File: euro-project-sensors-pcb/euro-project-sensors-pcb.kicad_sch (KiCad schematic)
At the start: 25 parts, among them J1 CH0, J2 CH0, J3 CH0, J4 CH0

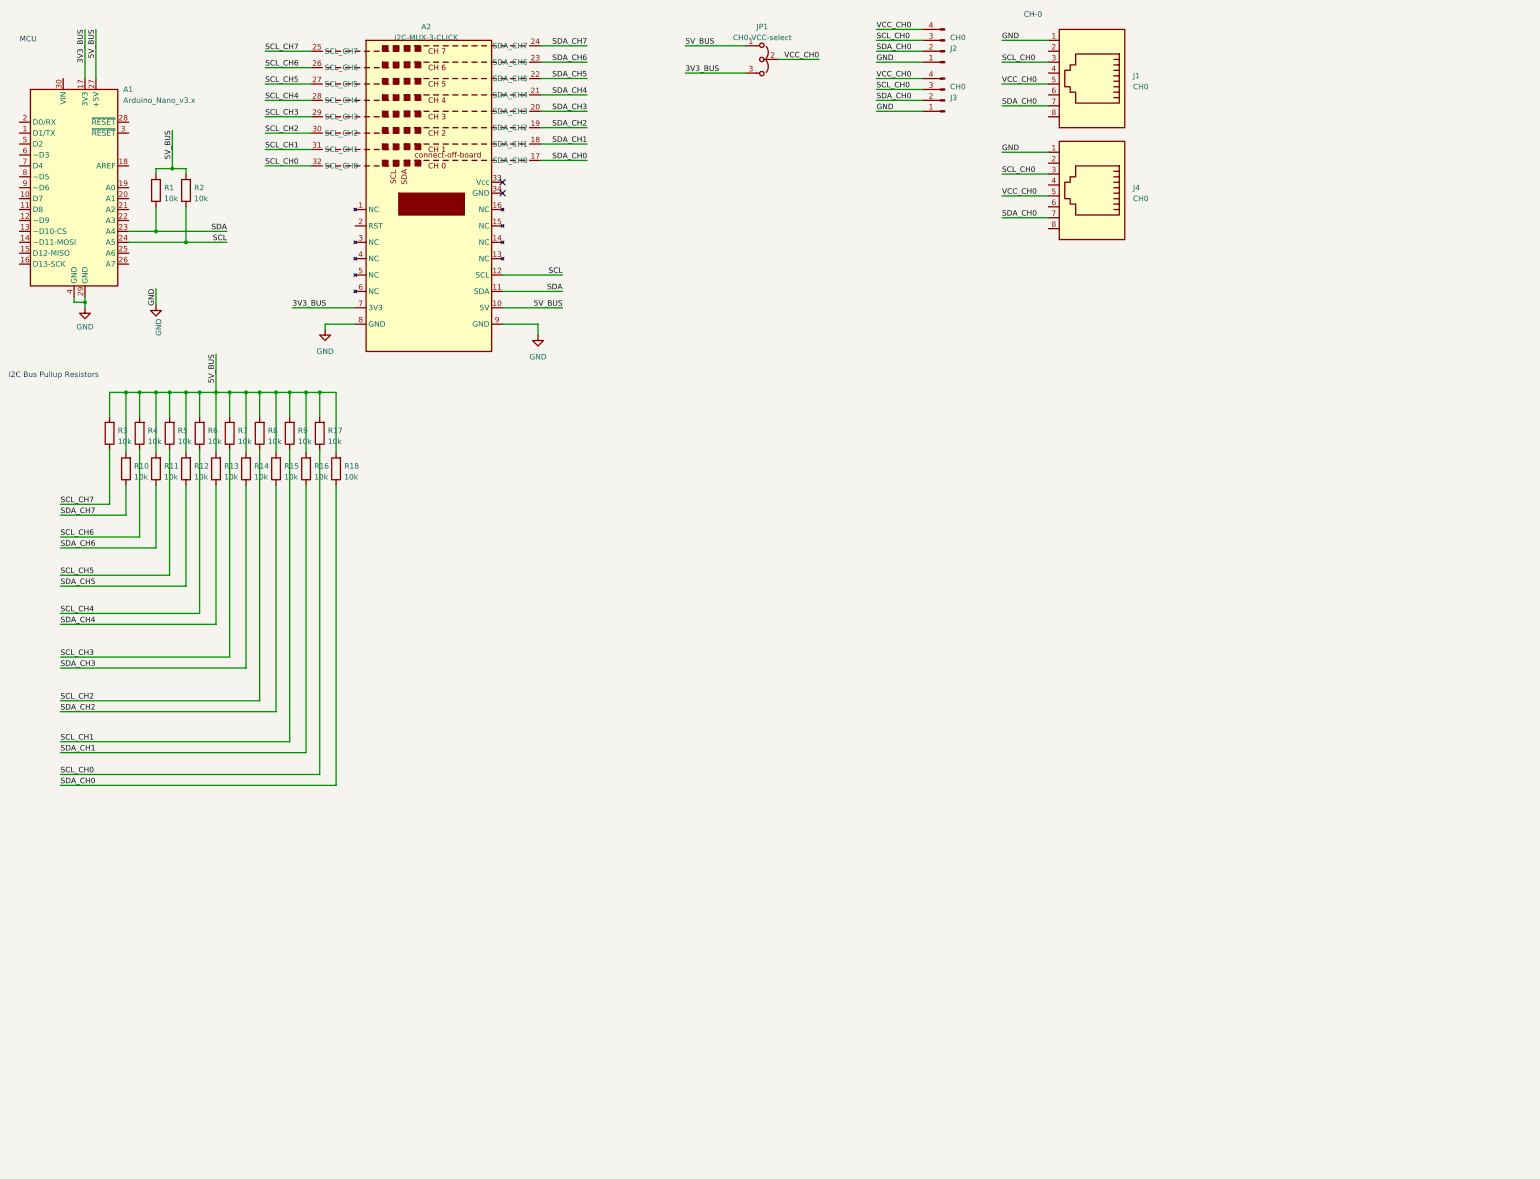
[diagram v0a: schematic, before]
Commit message: dfgbdfbdb
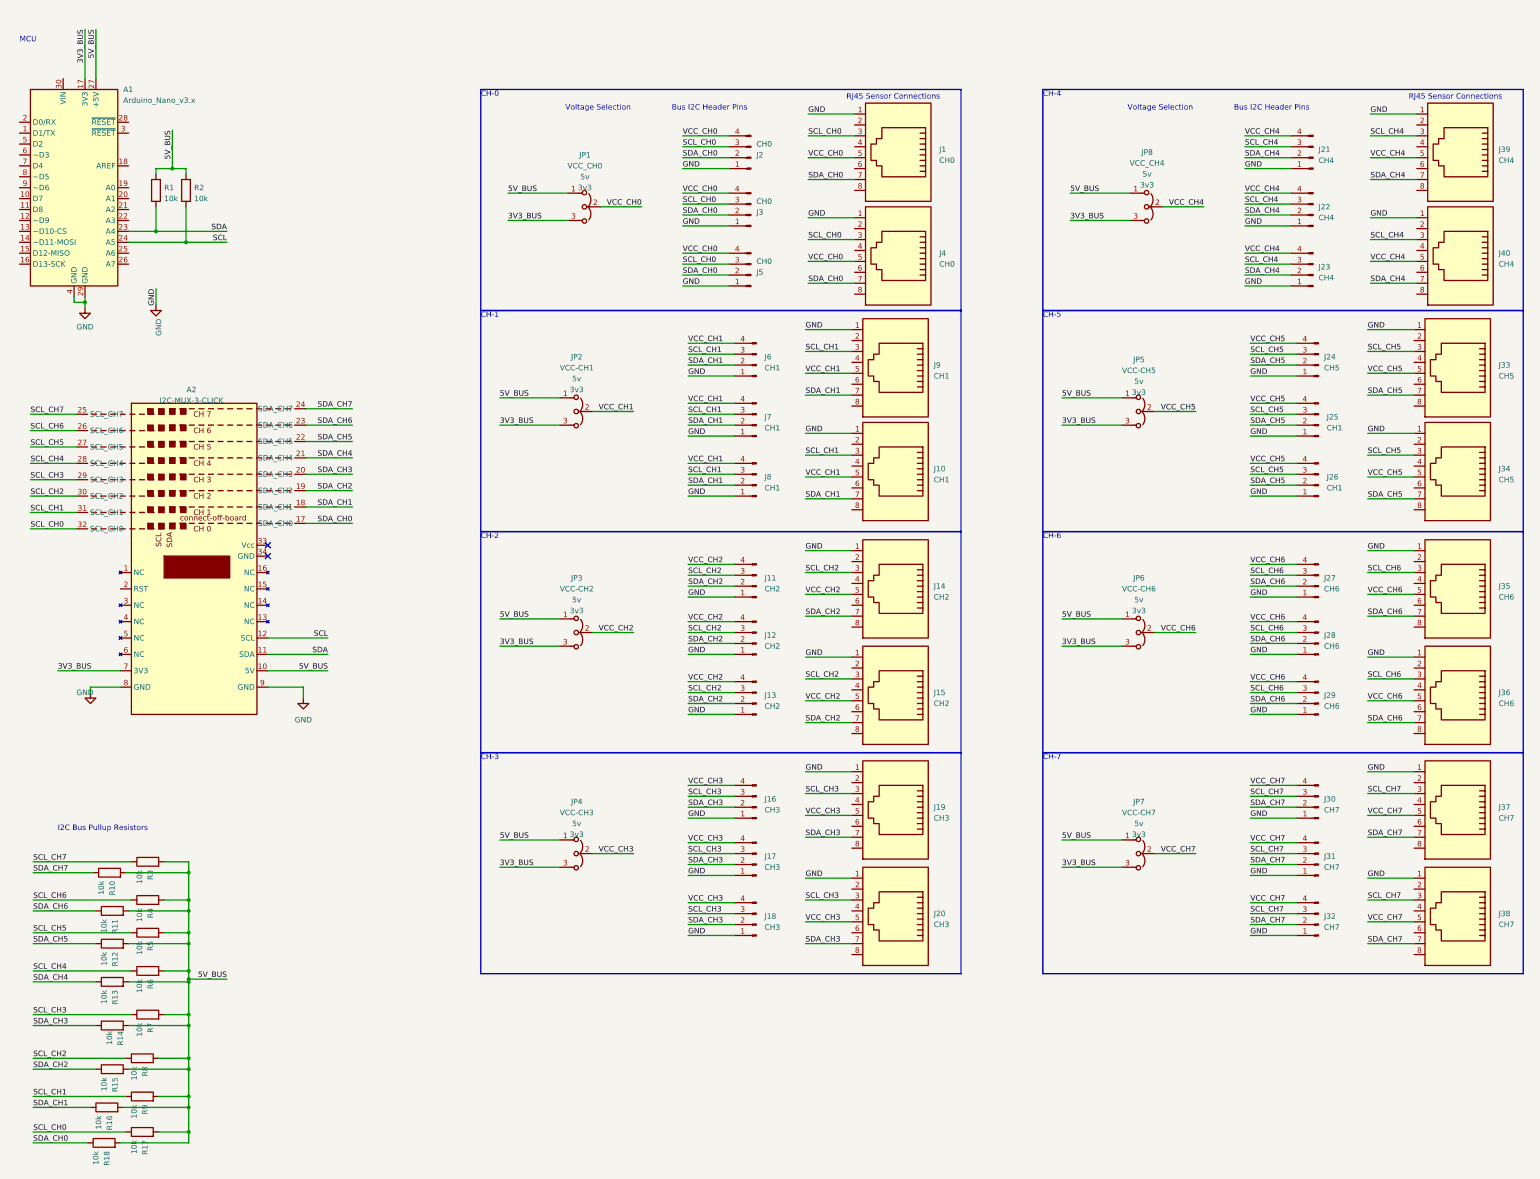
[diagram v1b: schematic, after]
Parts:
- added J10, J9: CH1, Connector_RJ:RJ45_OST_PJ012-8P8CX_Vertical, symbol Connector:RJ45
- added J11, J12, J13: CH2, Connector_PinHeader_2.54mm:PinHeader_1x04_P2.54mm_Vertical, symbol 000_Pin_Headers_Immo:Conn_01x04_Male
- added J14, J15: CH2, Connector_RJ:RJ45_OST_PJ012-8P8CX_Vertical, symbol Connector:RJ45
- added J16, J17, J18: CH3, Connector_PinHeader_2.54mm:PinHeader_1x04_P2.54mm_Vertical, symbol 000_Pin_Headers_Immo:Conn_01x04_Male
- added J19, J20: CH3, Connector_RJ:RJ45_OST_PJ012-8P8CX_Vertical, symbol Connector:RJ45
- added J21, J22, J23: CH4, Connector_PinHeader_2.54mm:PinHeader_1x04_P2.54mm_Vertical, symbol 000_Pin_Headers_Immo:Conn_01x04_Male
- added J24: CH5, Connector_PinHeader_2.54mm:PinHeader_1x04_P2.54mm_Vertical, symbol 000_Pin_Headers_Immo:Conn_01x04_Male
- added J25, J26, J6, J7, J8: CH1, Connector_PinHeader_2.54mm:PinHeader_1x04_P2.54mm_Vertical, symbol 000_Pin_Headers_Immo:Conn_01x04_Male
- added J27, J28, J29: CH6, Connector_PinHeader_2.54mm:PinHeader_1x04_P2.54mm_Vertical, symbol 000_Pin_Headers_Immo:Conn_01x04_Male
- added J30, J31, J32: CH7, Connector_PinHeader_2.54mm:PinHeader_1x04_P2.54mm_Vertical, symbol 000_Pin_Headers_Immo:Conn_01x04_Male
- added J33, J34: CH5, Connector_RJ:RJ45_OST_PJ012-8P8CX_Vertical, symbol Connector:RJ45
- added J35, J36: CH6, Connector_RJ:RJ45_OST_PJ012-8P8CX_Vertical, symbol Connector:RJ45
- added J37, J38: CH7, Connector_RJ:RJ45_OST_PJ012-8P8CX_Vertical, symbol Connector:RJ45
- added J39, J40: CH4, Connector_RJ:RJ45_OST_PJ012-8P8CX_Vertical, symbol Connector:RJ45
- added J5: CH0, Connector_PinHeader_2.54mm:PinHeader_1x04_P2.54mm_Vertical, symbol 000_Pin_Headers_Immo:Conn_01x04_Male
- added JP2: VCC-CH1, 000-jumpers-immo:SolderJumper-3-open-high-power, symbol 000-jumpers-immo:Jumper_3_Open3
- added JP3: VCC-CH2, 000-jumpers-immo:SolderJumper-3-open-high-power, symbol 000-jumpers-immo:Jumper_3_Open3
- added JP4: VCC-CH3, 000-jumpers-immo:SolderJumper-3-open-high-power, symbol 000-jumpers-immo:Jumper_3_Open3
- added JP5: VCC-CH5, 000-jumpers-immo:SolderJumper-3-open-high-power, symbol 000-jumpers-immo:Jumper_3_Open3
- added JP6: VCC-CH6, 000-jumpers-immo:SolderJumper-3-open-high-power, symbol 000-jumpers-immo:Jumper_3_Open3
- added JP7: VCC-CH7, 000-jumpers-immo:SolderJumper-3-open-high-power, symbol 000-jumpers-immo:Jumper_3_Open3
- added JP8: VCC_CH4, 000-jumpers-immo:SolderJumper-3-open-high-power, symbol 000-jumpers-immo:Jumper_3_Open3
- J2, J3: footprint Connector_PinHeader_1.27mm:PinHeader_1x04_P1.27mm_Vertical -> Connector_PinHeader_2.54mm:PinHeader_1x04_P2.54mm_Vertical
- JP1: value CH0-VCC-select -> VCC_CH0; footprint Jumper:SolderJumper-3_P1.3mm_Open_RoundedPad1.0x1.5mm_NumberLabels -> 000-jumpers-immo:SolderJumper-3-open-high-power; PIN_1 (none) -> 5v; PIN_3 (none) -> 3v3
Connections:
- net 3V3_BUS: now also JP2.3 (B), JP3.3 (B), JP4.3 (B), JP5.3 (B), JP6.3 (B), JP7.3 (B), JP8.3 (B)
- net 5V_BUS: now also JP2.1 (A), JP3.1 (A), JP4.1 (A), JP5.1 (A), JP6.1 (A), JP7.1 (A), JP8.1 (A)
- net GND: now also J10.1, J11.1 (Pin_1), J12.1 (Pin_1), J13.1 (Pin_1), J14.1, J15.1, J16.1 (Pin_1), J17.1 (Pin_1), J18.1 (Pin_1), J19.1, J20.1, J21.1 (Pin_1), J22.1 (Pin_1), J23.1 (Pin_1), J24.1 (Pin_1), J25.1 (Pin_1), J26.1 (Pin_1), J27.1 (Pin_1), J28.1 (Pin_1), J29.1 (Pin_1), J30.1 (Pin_1), J31.1 (Pin_1), J32.1 (Pin_1), J33.1, J34.1, J35.1, J36.1, J37.1, J38.1, J39.1, J40.1, J5.1 (Pin_1), J6.1 (Pin_1), J7.1 (Pin_1), J8.1 (Pin_1), J9.1
- net SCL_CH0: now also J5.3 (Pin_3)
- net SCL_CH1: now also J10.3, J6.3 (Pin_3), J7.3 (Pin_3), J8.3 (Pin_3), J9.3
- net SCL_CH2: now also J11.3 (Pin_3), J12.3 (Pin_3), J13.3 (Pin_3), J14.3, J15.3
- net SCL_CH3: now also J16.3 (Pin_3), J17.3 (Pin_3), J18.3 (Pin_3), J19.3, J20.3
- net SCL_CH4: now also J21.3 (Pin_3), J22.3 (Pin_3), J23.3 (Pin_3), J39.3, J40.3
- net SCL_CH5: now also J24.3 (Pin_3), J25.3 (Pin_3), J26.3 (Pin_3), J33.3, J34.3
- net SCL_CH6: now also J27.3 (Pin_3), J28.3 (Pin_3), J29.3 (Pin_3), J35.3, J36.3
- net SCL_CH7: now also J30.3 (Pin_3), J31.3 (Pin_3), J32.3 (Pin_3), J37.3, J38.3
- net SDA_CH0: now also J5.2 (Pin_2)
- net SDA_CH1: now also J10.7, J6.2 (Pin_2), J7.2 (Pin_2), J8.2 (Pin_2), J9.7
- net SDA_CH2: now also J11.2 (Pin_2), J12.2 (Pin_2), J13.2 (Pin_2), J14.7, J15.7
- net SDA_CH3: now also J16.2 (Pin_2), J17.2 (Pin_2), J18.2 (Pin_2), J19.7, J20.7
- net SDA_CH4: now also J21.2 (Pin_2), J22.2 (Pin_2), J23.2 (Pin_2), J39.7, J40.7
- net SDA_CH5: now also J24.2 (Pin_2), J25.2 (Pin_2), J26.2 (Pin_2), J33.7, J34.7
- net SDA_CH6: now also J27.2 (Pin_2), J28.2 (Pin_2), J29.2 (Pin_2), J35.7, J36.7
- net SDA_CH7: now also J30.2 (Pin_2), J31.2 (Pin_2), J32.2 (Pin_2), J37.7, J38.7
- net VCC_CH0: now also J5.4 (Pin_4)
- new net VCC_CH1: J10.5, J6.4 (Pin_4), J7.4 (Pin_4), J8.4 (Pin_4), J9.5, JP2.2 (C)
- new net VCC_CH2: J11.4 (Pin_4), J12.4 (Pin_4), J13.4 (Pin_4), J14.5, J15.5, JP3.2 (C)
- new net VCC_CH3: J16.4 (Pin_4), J17.4 (Pin_4), J18.4 (Pin_4), J19.5, J20.5, JP4.2 (C)
- new net VCC_CH4: J21.4 (Pin_4), J22.4 (Pin_4), J23.4 (Pin_4), J39.5, J40.5, JP8.2 (C)
- new net VCC_CH5: J24.4 (Pin_4), J25.4 (Pin_4), J26.4 (Pin_4), J33.5, J34.5, JP5.2 (C)
- new net VCC_CH6: J27.4 (Pin_4), J28.4 (Pin_4), J29.4 (Pin_4), J35.5, J36.5, JP6.2 (C)
- new net VCC_CH7: J30.4 (Pin_4), J31.4 (Pin_4), J32.4 (Pin_4), J37.5, J38.5, JP7.2 (C)
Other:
- note added: "Bus I2C Header Pins"
- note added: "CH-1"
- note added: "CH-2"
- note added: "CH-3"
- note added: "CH-4"
- note added: "CH-5"
- note added: "CH-6"
- note added: "CH-7"
- note added: "RJ45 Sensor Connections"
- note added: "Voltage Selection"
- moved on the sheet: A2, J1, J2, J3, J4, JP1, R10, R11, R12, R13, R14, R15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
